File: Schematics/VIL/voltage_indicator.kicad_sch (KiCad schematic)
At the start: 10 parts, among them Q1 VN2460, Q2 UJ3N120035K3S

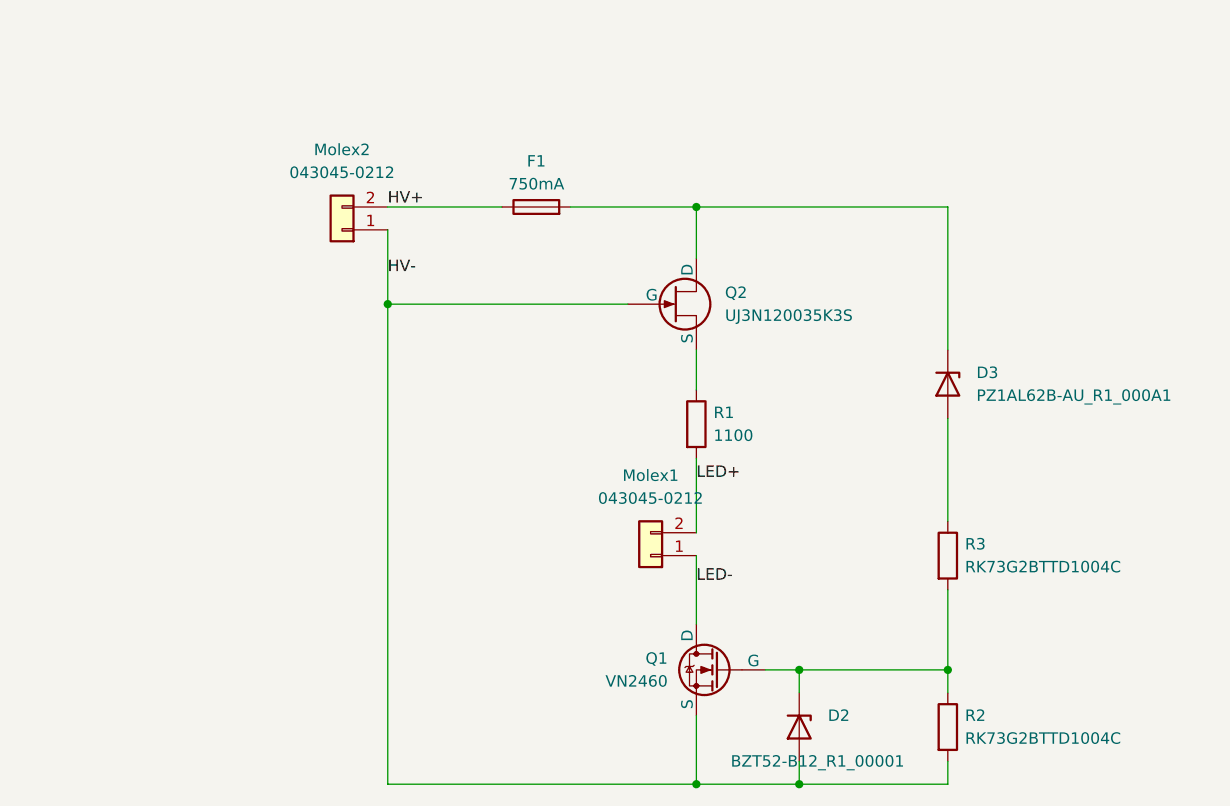
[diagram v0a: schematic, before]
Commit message: VIL edit
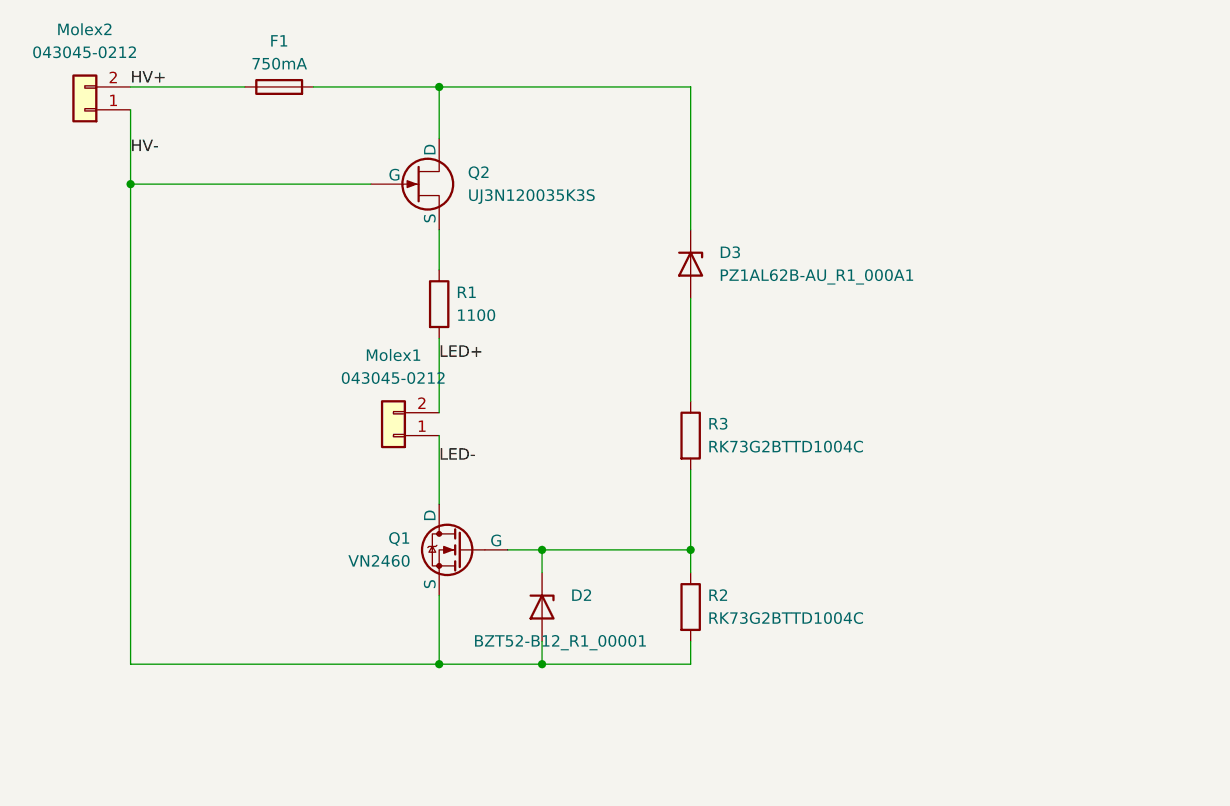
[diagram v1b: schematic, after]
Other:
- moved on the sheet: D2, D3, F1, Molex1, Molex2, Q1, Q2, R1, R2, R3
